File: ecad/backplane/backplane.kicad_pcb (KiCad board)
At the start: 2 copper layers, 160 x 220 mm, 22 parts, among them J1 10145891-0320J13LF, J2 10145891-0320J13LF, J3 USB4105-GF-A, J4 10145891-0320J13LF, J5 10145891-0320J13LF, J6 5017868090, U1 MCP16331x-xCH

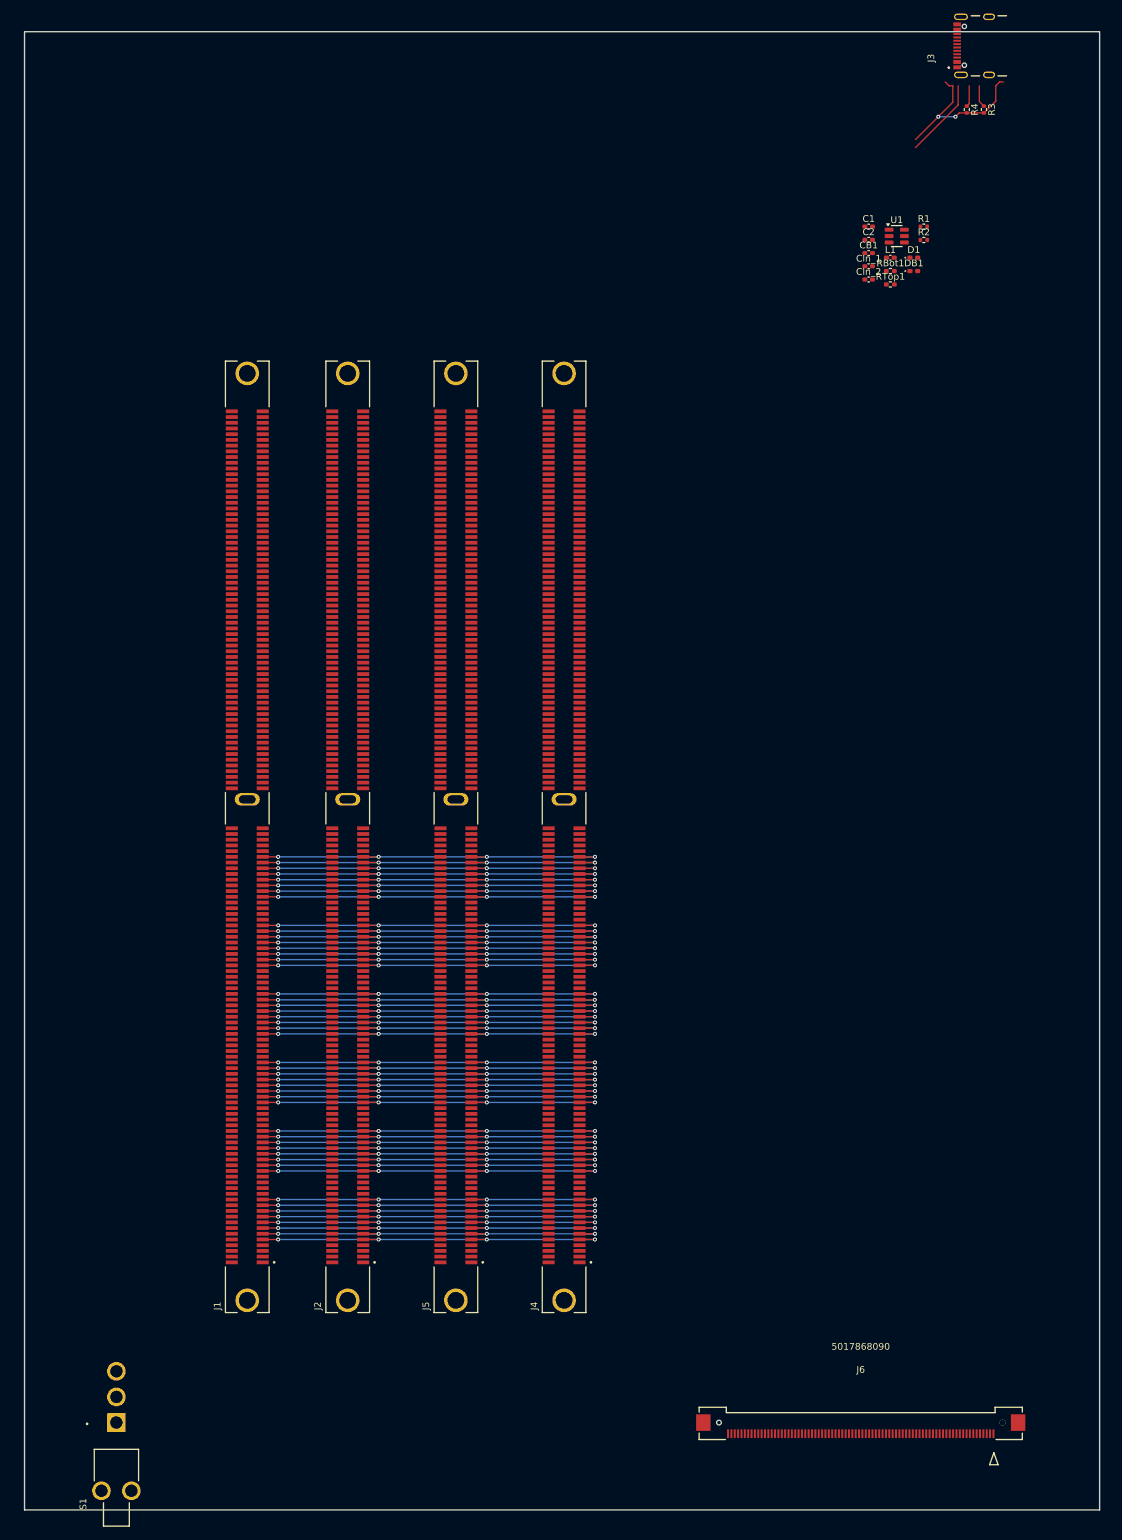
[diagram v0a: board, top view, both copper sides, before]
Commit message: backplane with addr
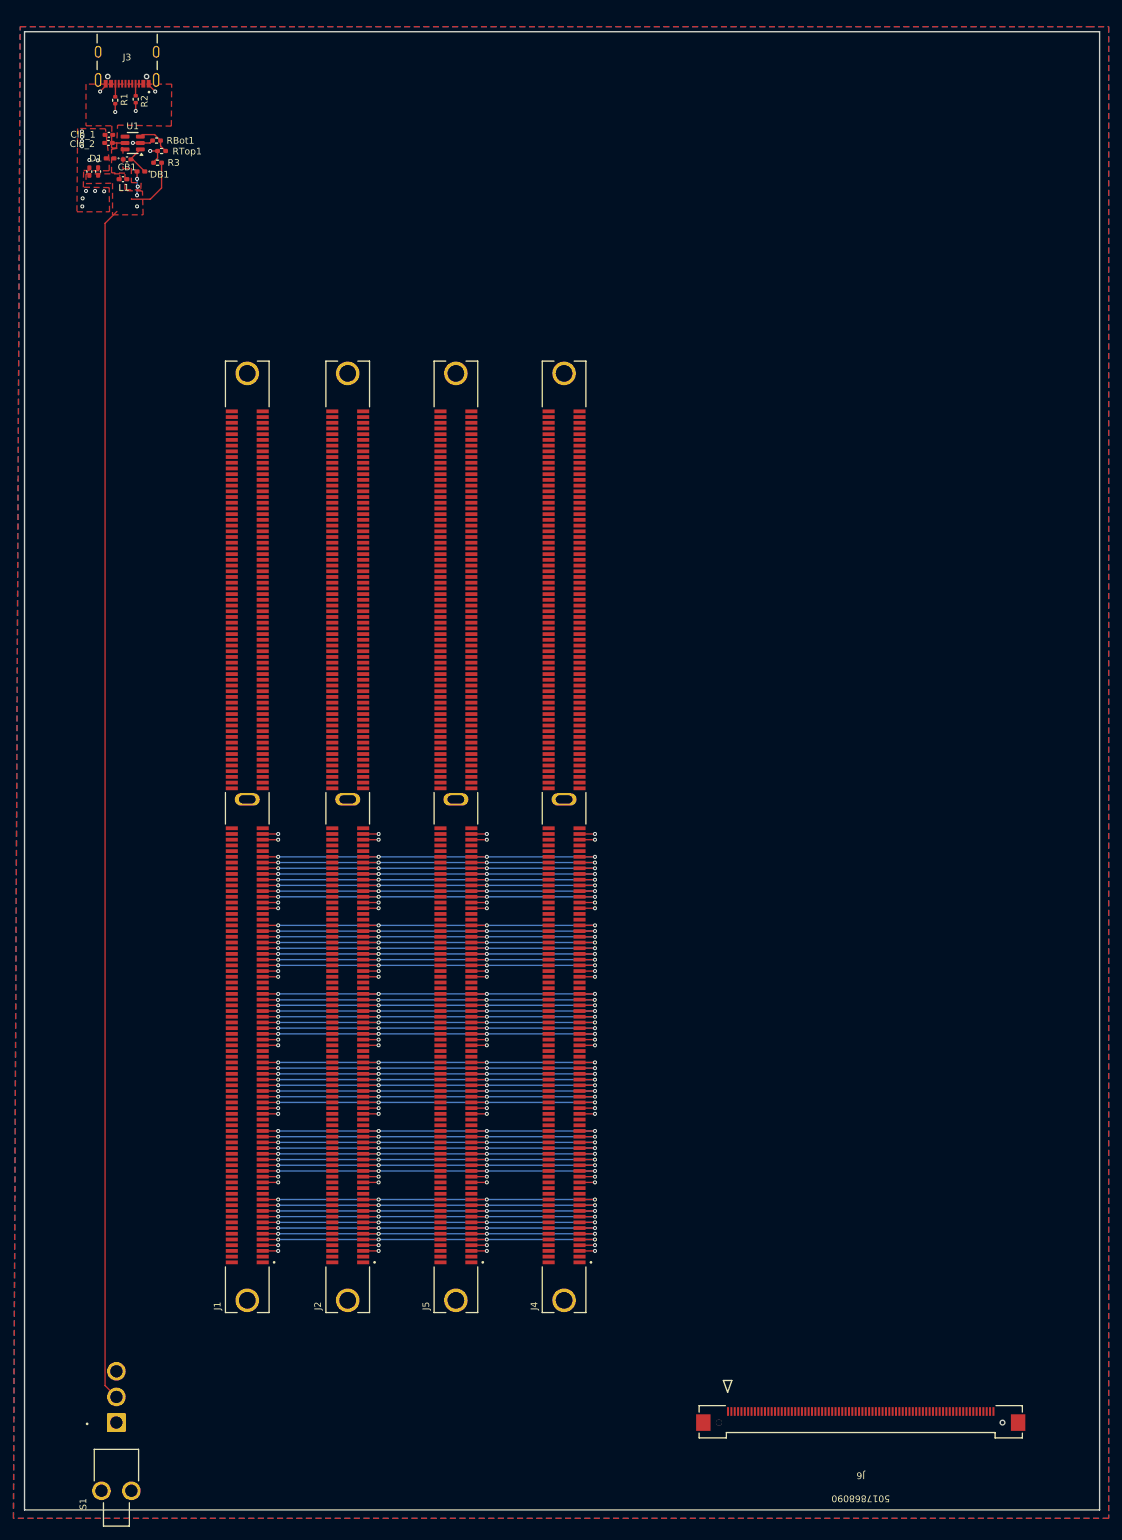
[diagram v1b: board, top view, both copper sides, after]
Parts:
- removed R4: 5.1k, Resistor_SMD:R_0402_1005Metric
- R3: value 5.1k -> 10; footprint Resistor_SMD:R_0402_1005Metric -> Resistor_SMD:R_0402_1005Metric_Pad0.72x0.64mm_HandSolder
- moved J3 128.3 mm to (87.9, 35.7), turned to 180 degrees
- moved R3 123.2 mm to (92.5, 52.2), turned to 0 degrees
- moved R1 121.8 mm to (86.2, 43.0), turned to -90 degrees
- moved D1 120.5 mm to (85.4, 51.6), turned to 180 degrees
- moved R2 119.1 mm to (89.2, 42.8), turned to -90 degrees
- moved C1 116.3 mm to (82.3, 53.6), turned to 90 degrees
- moved DB1 116.0 mm to (90.0, 53.5), turned to 180 degrees
- moved C2 115.1 mm to (83.6, 53.5), turned to 90 degrees
- moved Cln_2 114.9 mm to (85.2, 49.3), turned to 180 degrees
- moved L1 114.8 mm to (87.3, 54.7), turned to 180 degrees
- moved Cln_1 114.8 mm to (85.2, 48.1), turned to 180 degrees
- moved U1 114.6 mm to (88.8, 49.3), turned to 180 degrees
- moved CB1 111.3 mm to (87.9, 51.8), turned to 180 degrees
- moved RBot1 110.9 mm to (92.3, 49.0), turned to 180 degrees
- moved RTop1 110.3 mm to (93.0, 50.5), turned to 180 degrees
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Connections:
- net +5V renamed VBUS
- CB1 pad 2: Net-(U1-BOOST) -> Net-(D1-K)
- J3 pad A5: unconnected-(J3-CC1-PadA5) -> Net-(J3-CC1)
- J3 pad B5: unconnected-(J3-CC2-PadB5) -> Net-(J3-CC2)
- J3 pad B6: Net-(J3-DP2) -> unconnected-(J3-DP2-PadB6)
- J3 pad B7: Net-(J3-DN2) -> unconnected-(J3-DN2-PadB7)
- R1 pad 1: Net-(J3-DN2) -> Net-(J3-CC2)
- R2 pad 1: Net-(J3-DP2) -> Net-(J3-CC1)
- R3 pad 1: Net-(J6-DN2) -> Net-(R3-Pad1)
- R3 pad 2: GND -> 3.3V IN
- RTop1 pad 2: 3.3V IN -> Net-(R3-Pad1)
- U1 pad 1: Net-(U1-BOOST) -> Net-(DB1-K)
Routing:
- net 3.3V IN: track 0.00 -> 190.4 mm, vias 0 -> 3
- net GND: track 24.8 -> 137.3 mm, vias 2 -> 72
- net VBUS: track 11.8 -> 1.90 mm
- net Net-(U1-V_{FB}): track 0.00 -> 5.36 mm
- net Net-(DB1-K): track 0.00 -> 5.11 mm
- net Net-(J6-DN2): track 3.30 -> 0.00 mm
- net Net-(J6-DP2): track 3.17 -> 0.00 mm
- net Net-(R3-Pad1): track 0.00 -> 3.00 mm, vias 0 -> 1
- net Net-(J3-CC2): track 0.00 -> 1.96 mm
- net Net-(J3-CC1): track 0.00 -> 1.81 mm
- net Net-(D1-K): vias 0 -> 1
- added copper zone on F.Cu, net 3.3V
- added copper zone on F.Cu, net 3.3V IN
- added copper zone on B.Cu, net GND
- added copper zone on F.Cu, net GND
- added copper zone on F.Cu, net Net-(D1-K)
- added copper zone on F.Cu, net VBUS
